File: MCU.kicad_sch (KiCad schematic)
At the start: 9 parts, among them U1 NRF52832-QFAB-R, Y1 32.768kHz

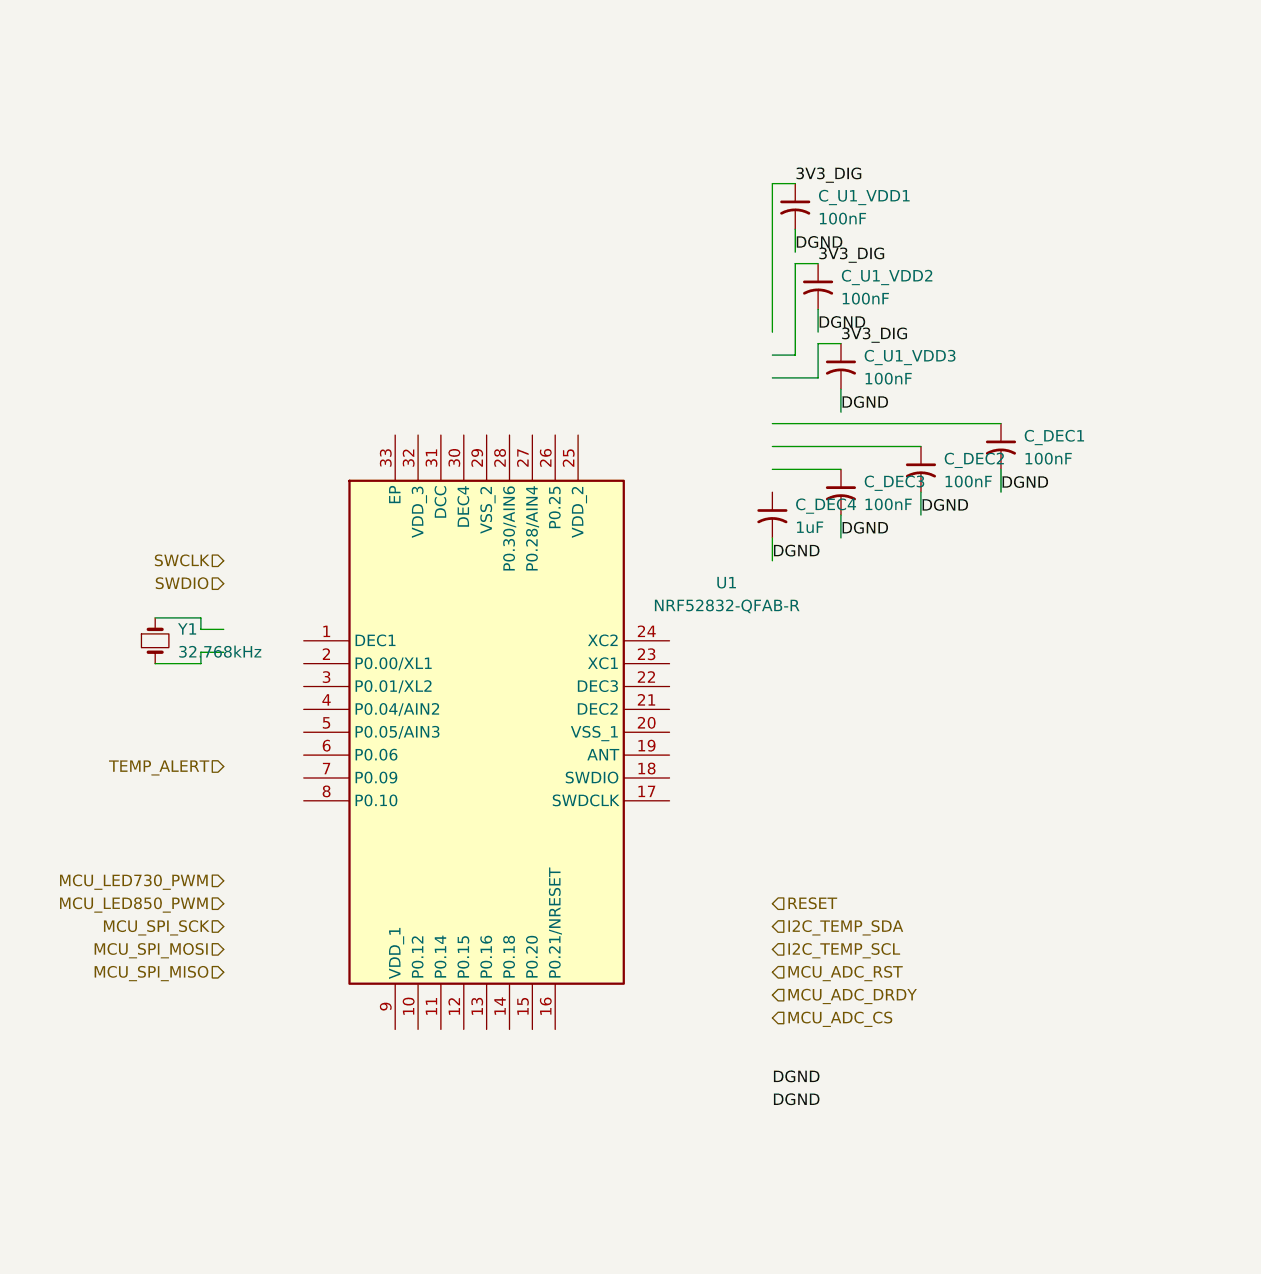
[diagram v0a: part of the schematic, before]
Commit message: mcu ready except antenna
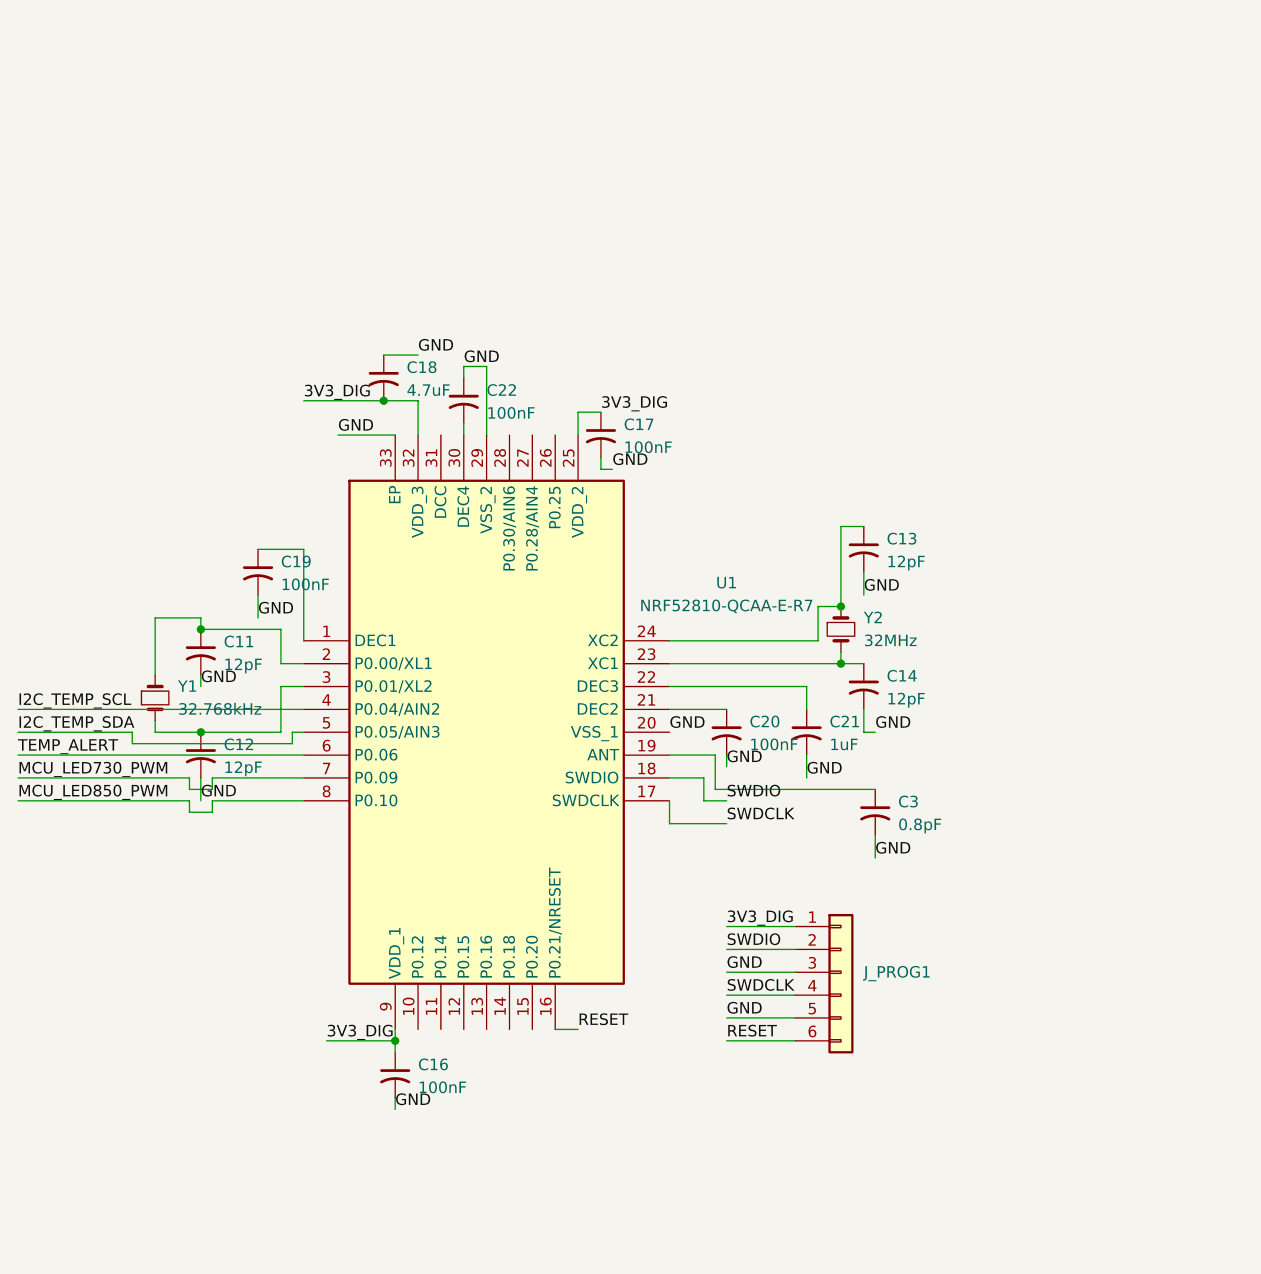
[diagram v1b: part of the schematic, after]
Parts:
- removed C_DEC3: 100nF, symbol Device:C_Small_US
- removed C_DEC4: 1uF, symbol Device:C_Small_US
- added C11, C12, C13, C14: 12pF, symbol Device:C_Small_US
- added C16: 100nF, symbol Device:C_Small_US
- added C18: 4.7uF, symbol Device:C_Small_US
- added C3: 0.8pF, symbol Device:C_Small_US
- added J_PROG1: TC2030-IDC-NL, TC2030-IDC-NL, symbol Connector_Generic:Conn_01x06
- added Y2: 32MHz, symbol Device:Crystal_Small
- C21: renamed from C_U1_VDD3; value 100nF -> 1uF
- U1: value NRF52832-QFAB-R -> NRF52810-QCAA-E-R7
- renumbered C_U1_VDD1 to C17, C_DEC1 to C19, C_U1_VDD2 to C20, C_DEC2 to C22
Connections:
- net 3V3_DIG: now also U1.25 (VDD_2), U1.32 (VDD_3), U1.9 (VDD_1), C16.1, C18.2, J_PROG1.1 (Pin_1); no longer C20.1, C21.1
- net I2C_TEMP_SCL: now also U1.4 (P0.04/AIN2)
- net I2C_TEMP_SDA: now also U1.5 (P0.05/AIN3)
- net MCU_LED730_PWM: now also U1.7 (P0.09)
- net MCU_LED850_PWM: now also U1.8 (P0.10)
- net RESET: now also U1.16 (P0.21/NRESET), J_PROG1.6 (Pin_6)
- net SWDIO: now also U1.18 (SWDIO), J_PROG1.2 (Pin_2)
- net TEMP_ALERT: now also U1.6 (P0.06)
- net at Y1.1: now also U1.2 (P0.00/XL1), C11.1
- net at Y1.2: now also U1.3 (P0.01/XL2), C12.1
- net at U1.1 (DEC1): now also C19.1
- net SWDCLK: now reaches U1.17 (SWDCLK)
- net SWDCLK: now also J_PROG1.4 (Pin_4)
- net at U1.19 (ANT): now also C3.1
- net GND: now reaches U1.20 (VSS_1)
- net GND: now also C17.2, C19.2, C20.2, C21.2, C22.1, U1.29 (VSS_2), U1.33 (EP), C11.2, C12.2, C13.2, C14.2, C16.2, C18.1, C3.2, J_PROG1.3 (Pin_3), J_PROG1.5 (Pin_5)
- net at U1.21 (DEC2): now also C20.1
- net at U1.22 (DEC3): now also C21.1
- net at U1.23 (XC1): now also C14.1, Y2.2
- net at U1.24 (XC2): now also C13.1, Y2.1
- net at U1.30 (DEC4): now also C22.2
- removed net DGND: C17.2, C19.2, C20.2, C21.2, C22.2
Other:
- moved on the sheet: C17, C19, C20, C21, C22, Y1
